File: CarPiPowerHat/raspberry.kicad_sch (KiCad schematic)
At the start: 6 parts, among them J9 40HAT, U4 CAT24C32

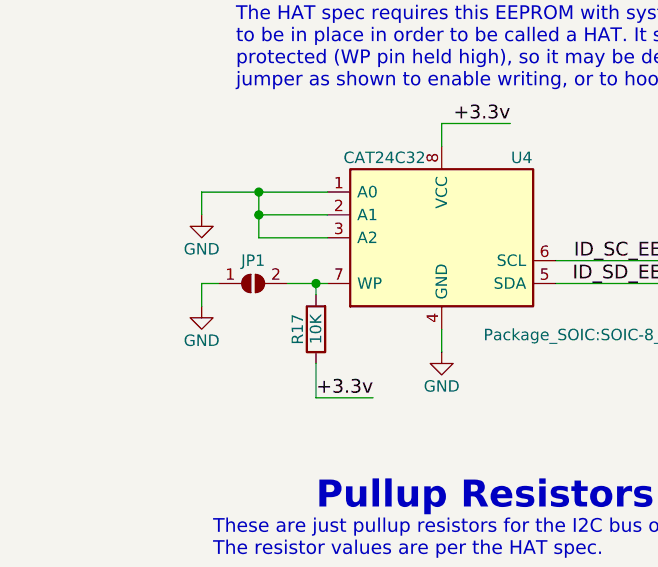
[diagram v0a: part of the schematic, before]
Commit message: Some bugfixing, added cam.py script
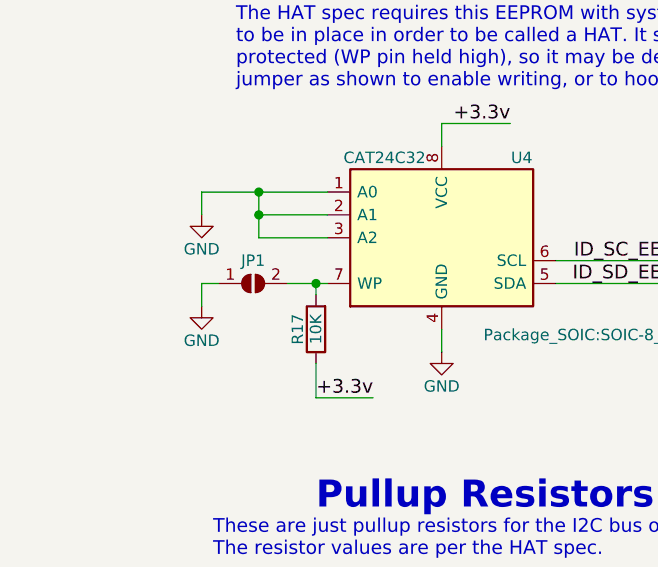
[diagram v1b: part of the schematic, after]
